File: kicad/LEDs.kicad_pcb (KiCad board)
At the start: 2 copper layers, 27.9 x 63.5 mm, 18 parts, among them J1 24V, J2 FTDI 3.3v, J3 24V, RGB, Q1 IRLZ44N, Q2 IRLZ44N, Q3 IRLZ44N, SW1 Reset, SW2 Flash Enable, U1 LM317_SOT-223, U2 ESP-12F

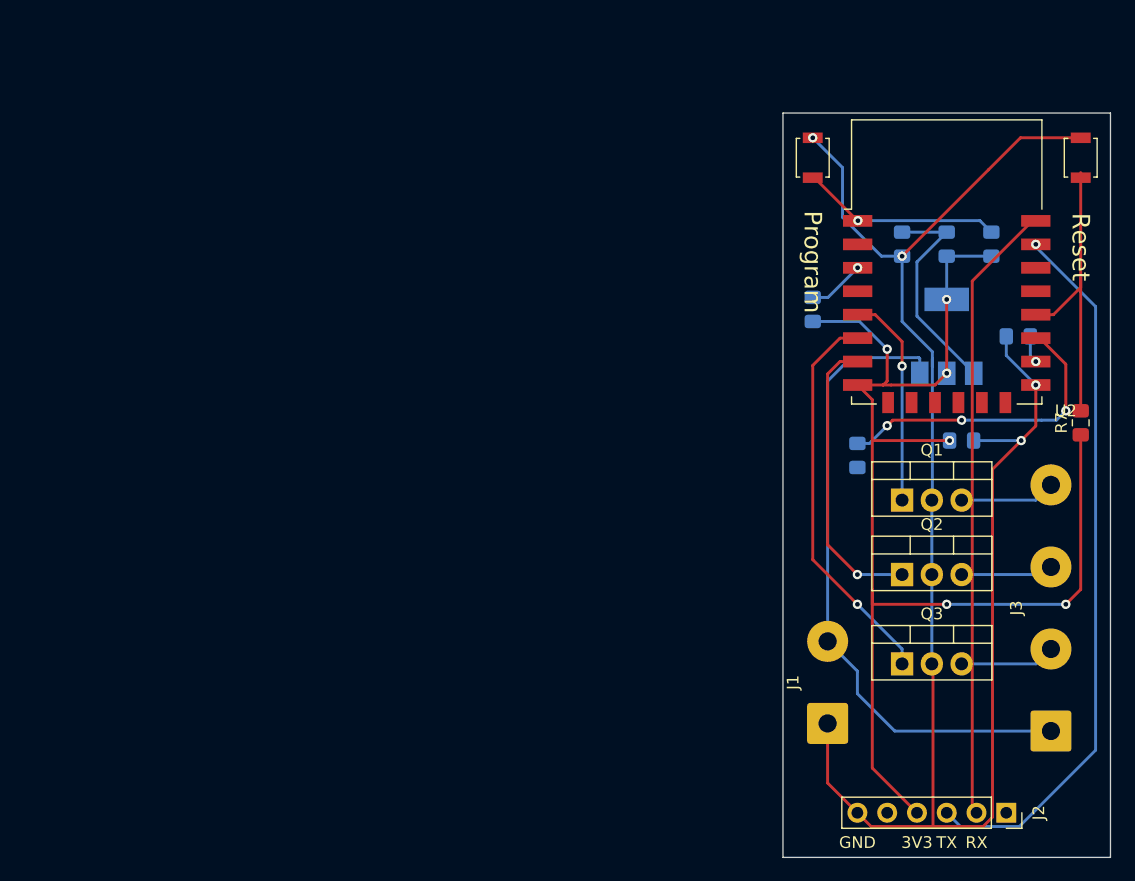
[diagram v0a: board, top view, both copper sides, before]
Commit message: More organized board
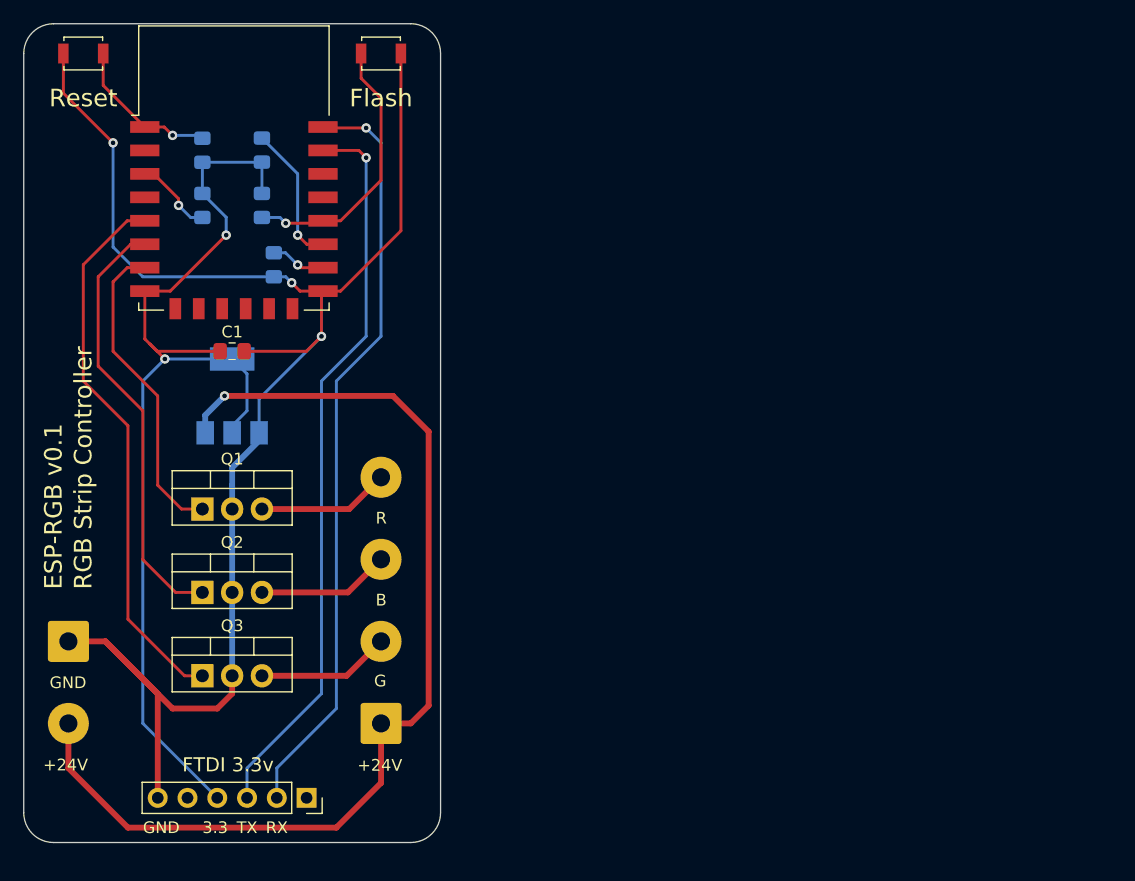
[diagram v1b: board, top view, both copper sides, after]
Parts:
- removed R1: 200, Resistor_SMD:R_0805_2012Metric_Pad1.15x1.40mm_HandSolder
- removed R2: 330, Resistor_SMD:R_0805_2012Metric_Pad1.15x1.40mm_HandSolder
- C1: moved to F.Cu
- R7: moved to B.Cu
- SW2: value Flash Enable -> Flash
- U1: value LM317_SOT-223 -> LM1117-3.3
- moved R7 72.3 mm to (149.9, 52.3), turned to 270 degrees
- moved R3 67.8 mm to (144.8, 47.6)
- moved J1 65.1 mm to (133.3, 89.5), turned to 270 degrees
- moved R6 63.8 mm to (150.9, 57.4), turned to 270 degrees
- moved SW1 62.9 mm to (134.6, 39.4), turned to 0 degrees
- moved C1 62.7 mm to (147.3, 64.8)
- moved U2 61.3 mm to (147.5, 49.1)
- moved U1 61.2 mm to (147.3, 68.6)
- moved SW2 60.3 mm to (160.0, 39.4), turned to 0 degrees
- moved Q2 59.7 mm to (144.8, 85.3)
- moved J2 59.7 mm to (153.7, 102.9)
- moved Q3 59.7 mm to (144.8, 92.5)
- moved Q1 59.7 mm to (144.8, 78.2)
- moved J3 57.2 mm to (160.0, 96.5)
- moved R5 57.1 mm to (149.9, 47.6)
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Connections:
- U1 pad 1: Net-(R1-Pad2) -> Net-(C1-Pad2)
- U2 pad 5: Net-(Q1-Pad1) -> Net-(Q3-Pad1)
- U2 pad 6: Net-(Q3-Pad1) -> Net-(Q2-Pad1)
- U2 pad 7: Net-(Q2-Pad1) -> Net-(Q1-Pad1)
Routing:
- net Net-(J1-Pad2): track 55.5 -> 89.8 mm, vias 0 -> 1
- net Net-(C1-Pad1): track 110.8 -> 90.4 mm, vias 6 -> 2
- net Net-(R1-Pad2): track 19.0 -> 0.00 mm
- net Net-(C1-Pad2): track 152.8 -> 138.4 mm, vias 4 -> 3
- net Net-(R5-Pad2): track 26.4 -> 12.0 mm, vias 3 -> 1
- net Net-(Q3-Pad1): track 33.4 -> 47.0 mm, vias 1 -> 0
- net Net-(Q2-Pad1): track 25.0 -> 37.1 mm, vias 1 -> 0
- net Net-(J2-Pad2): track 53.1 -> 65.1 mm, vias 0 -> 1
- net Net-(Q1-Pad1): track 18.3 -> 26.8 mm, vias 1 -> 0
- net Net-(R3-Pad2): track 17.2 -> 13.0 mm
- net Net-(J3-Pad3): track 7.89 -> 11.3 mm
- net Net-(J3-Pad2): track 8.15 -> 11.4 mm
- net Net-(J3-Pad4): track 8.16 -> 11.3 mm
- net Net-(R7-Pad2): track 26.0 -> 23.4 mm, vias 0 -> 1
- net Net-(R6-Pad1): track 2.37 -> 4.72 mm
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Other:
- board size 27.9 x 63.5 mm -> 35.6 x 69.9 mm
- board text added: "+24V"
- board text added: "3.3"
- board text added: "B"
- board text added: "ESP-RGB v0.1"
- board text added: "G"
- board text added: "R"
- board text added: "RGB Strip Controller"
- board text added: "pta2002.com"
- board text removed: "3V3"
- board text removed: "Program"
- board text removed: "RGB LED ESP8266"
- board text removed: "Reset"
